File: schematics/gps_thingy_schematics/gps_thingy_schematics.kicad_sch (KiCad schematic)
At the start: 4 parts, among them J1 Conn_01x04, J2 Conn_01x01, J3 Conn_01x06, J4 Conn_01x04

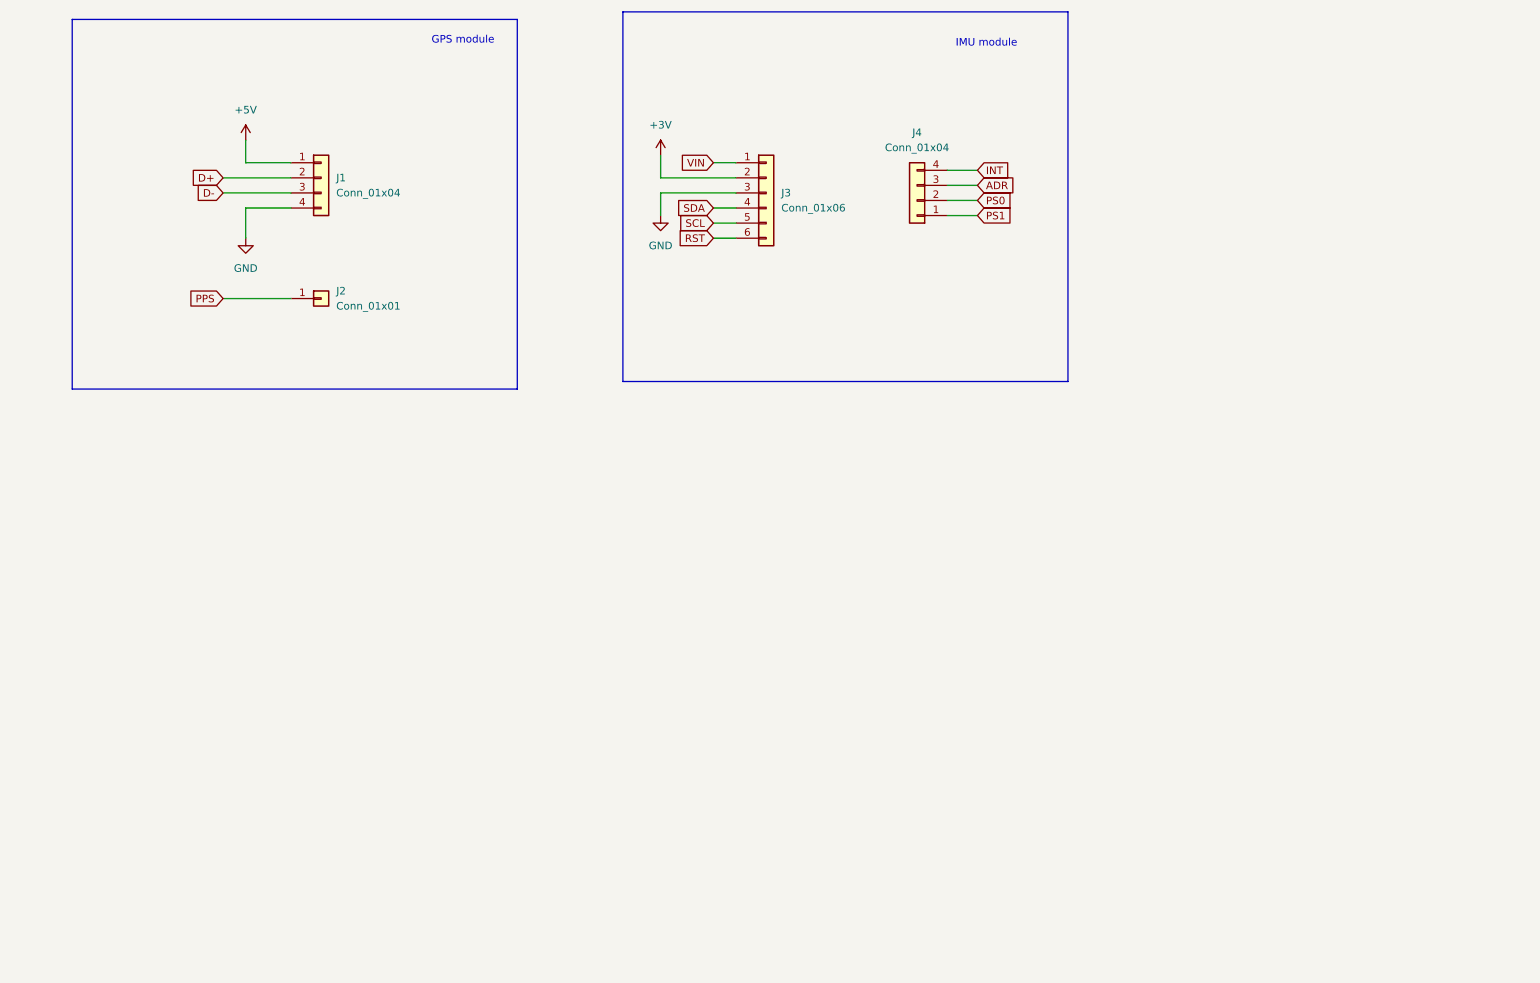
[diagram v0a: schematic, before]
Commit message: finishing schematics
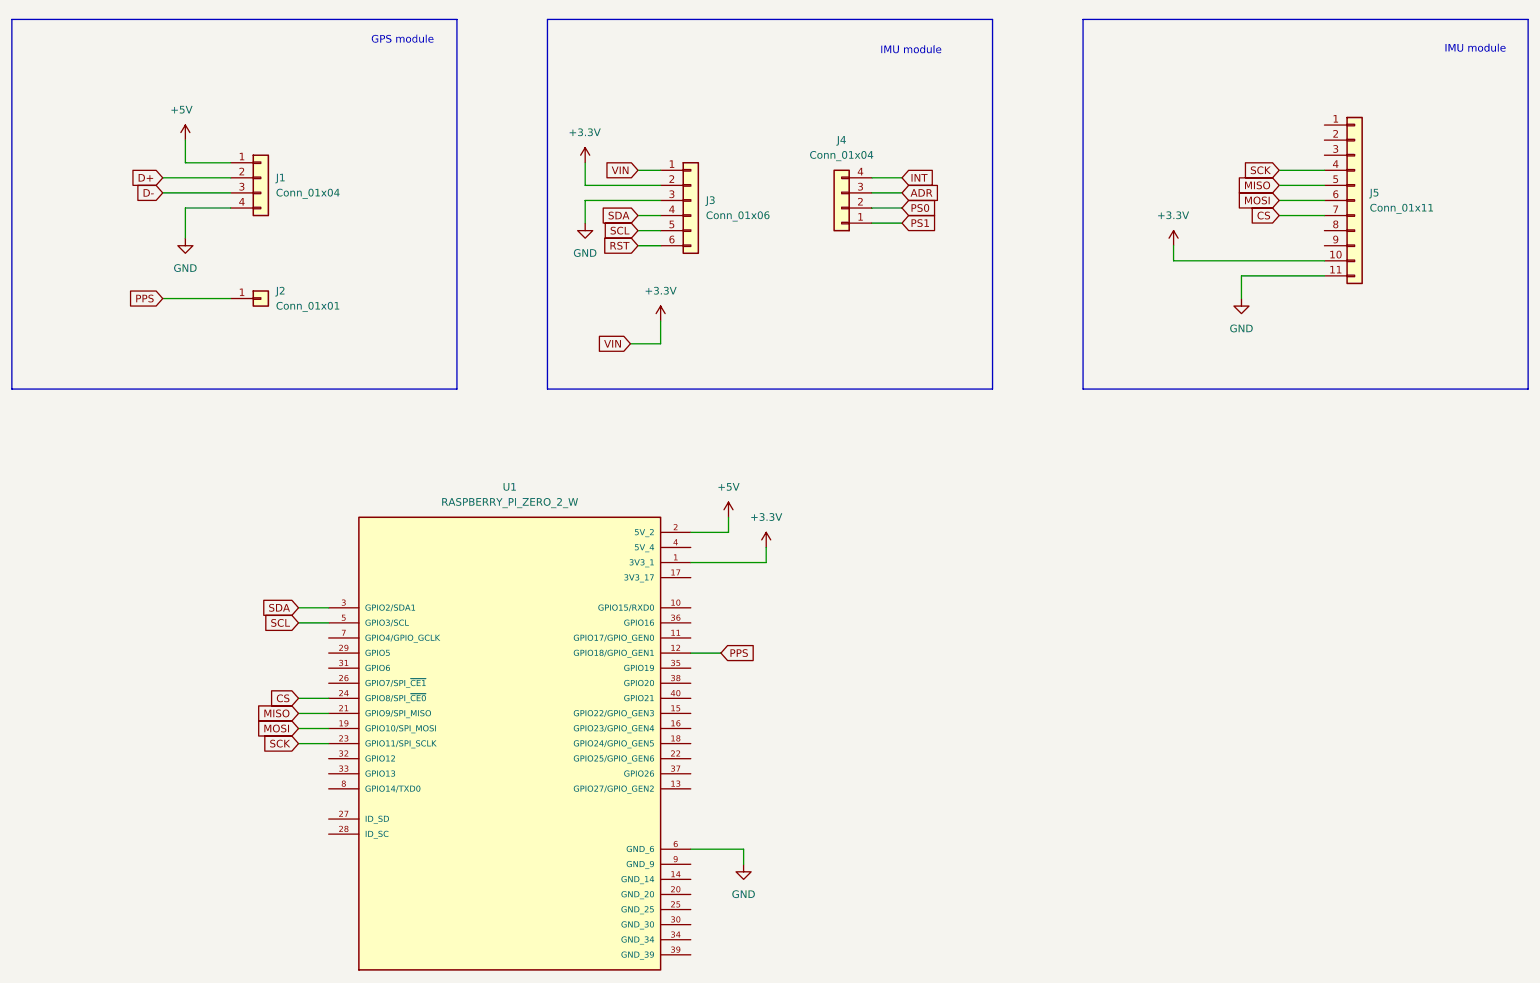
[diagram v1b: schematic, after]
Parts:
- added J5: Conn_01x11, symbol Connector_Generic:Conn_01x11
- added U1: RASPBERRY_PI_ZERO_2_W, RASPBERRY_PI_ZERO_2_W:MODULE_RASPBERRY_PI_ZERO_2_W, symbol rapi:RASPBERRY_PI_ZERO_2_W
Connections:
- net VIN is gone; now on net +3.3V: J3.1 (Pin_1)
- net +5V: now also U1.2 (5V_2)
- net GND: now also J5.11 (Pin_11), U1.6 (GND_6)
- net PPS: now also U1.12 (GPIO18/GPIO_GEN1)
- net SCL: now also U1.5 (GPIO3/SCL)
- net SDA: now also U1.3 (GPIO2/SDA1)
- net +3V renamed +3.3V
- net +3.3V: now also J5.10 (Pin_10), U1.1 (3V3_1)
- new net CS: J5.7 (Pin_7), U1.24 (GPIO8/SPI_~{CE0})
- new net MISO: J5.5 (Pin_5), U1.21 (GPIO9/SPI_MISO)
- new net MOSI: J5.6 (Pin_6), U1.19 (GPIO10/SPI_MOSI)
- new net SCK: J5.4 (Pin_4), U1.23 (GPIO11/SPI_SCLK)
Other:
- moved on the sheet: J1, J2, J3, J4
